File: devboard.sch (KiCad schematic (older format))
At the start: 112 parts, among them J1 USB_B, K1 HF3FA-012-ZTF, K2 HF3FA-012-ZTF

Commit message: Switches and buttons finished
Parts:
- added J?: Switches, symbol Connector_Generic:Conn_01x08
- K1, K2, K?: symbol hello-there:HF3FA-012-ZTF -> devboard-rescue:HF3FA-012-ZTF-hello-there
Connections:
- net S1: now also J?.1 (Pin_1)
- net S2: now also J?.2 (Pin_2)
- net S3: now also J?.3 (Pin_3)
- net S4: now also J?.4 (Pin_4)
- net S5: now also J?.5 (Pin_5)
- net S6: now also J?.6 (Pin_6)
- net S7: now also J?.7 (Pin_7)
- net S8: now also J?.8 (Pin_8)
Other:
- note added: "Switches"
- moved on the sheet: C?, R?, SW?

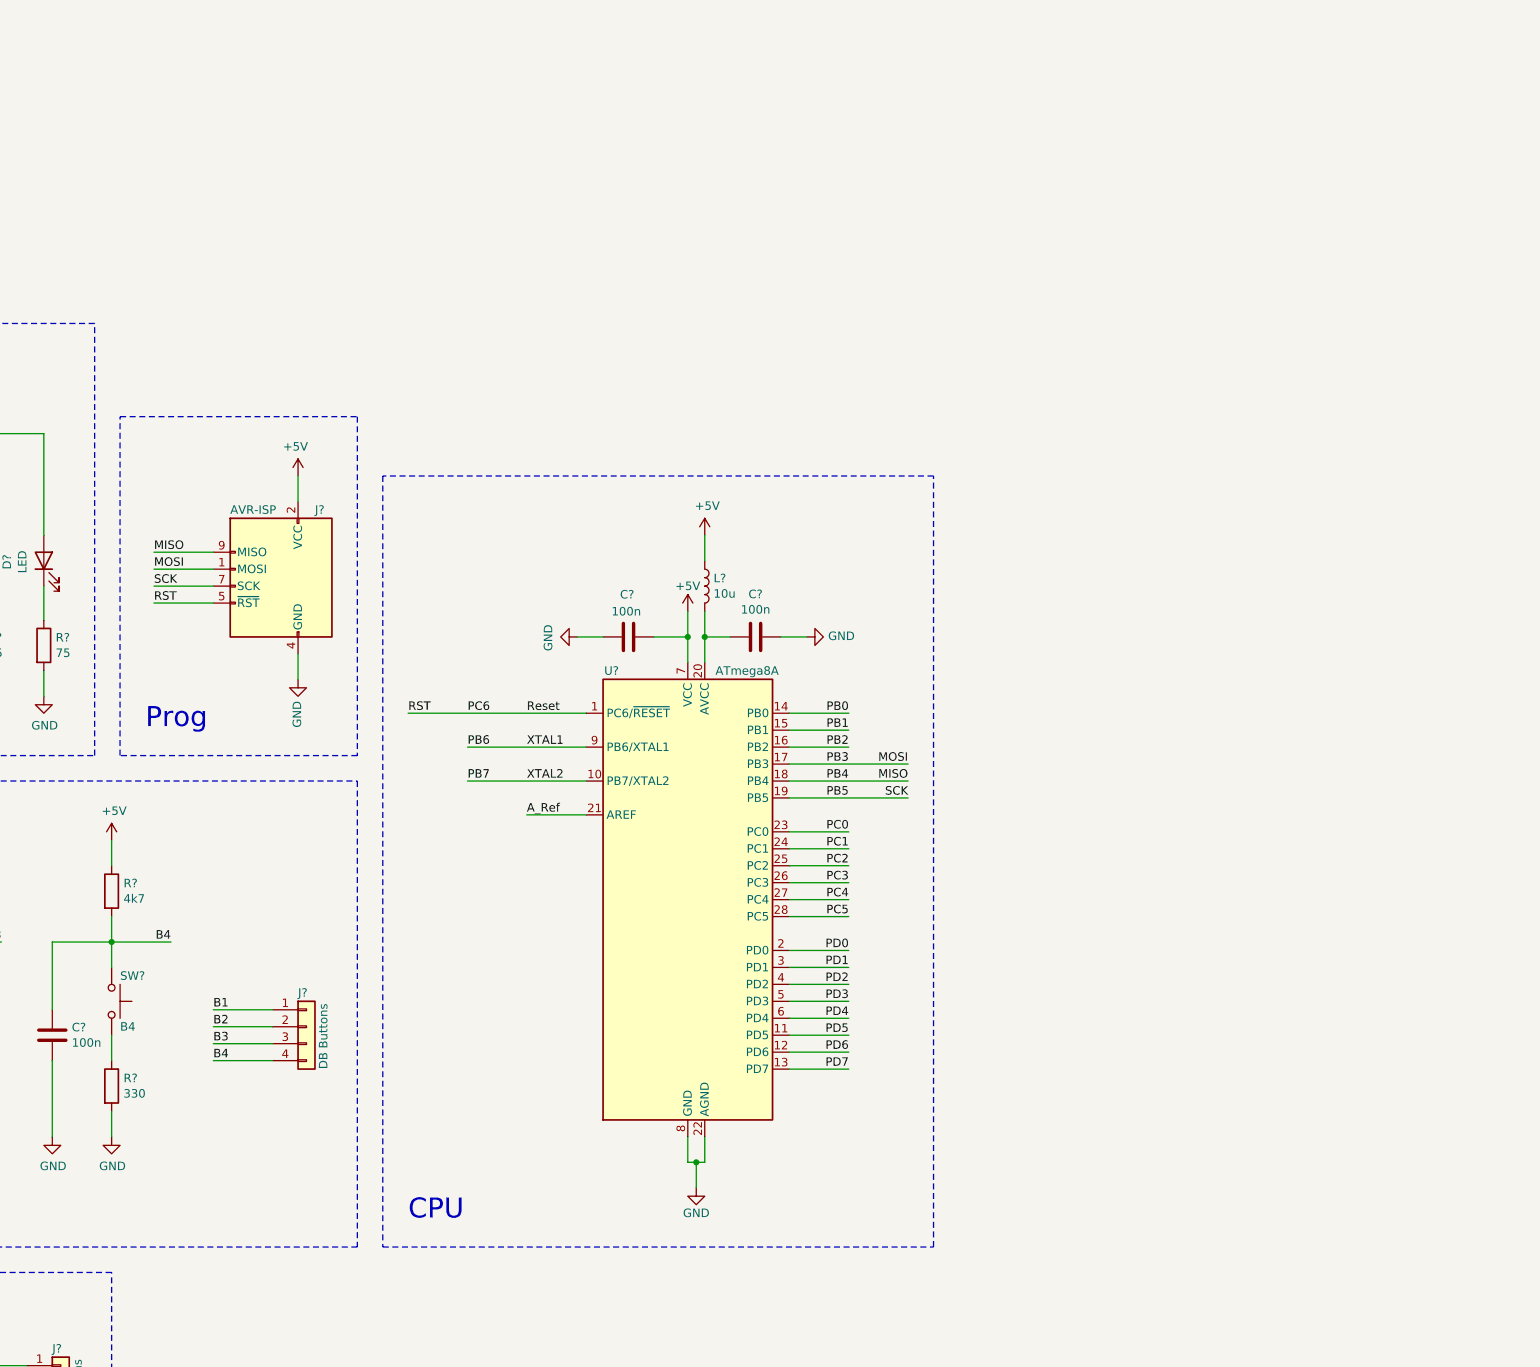
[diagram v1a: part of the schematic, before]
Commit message: Pots + rgb
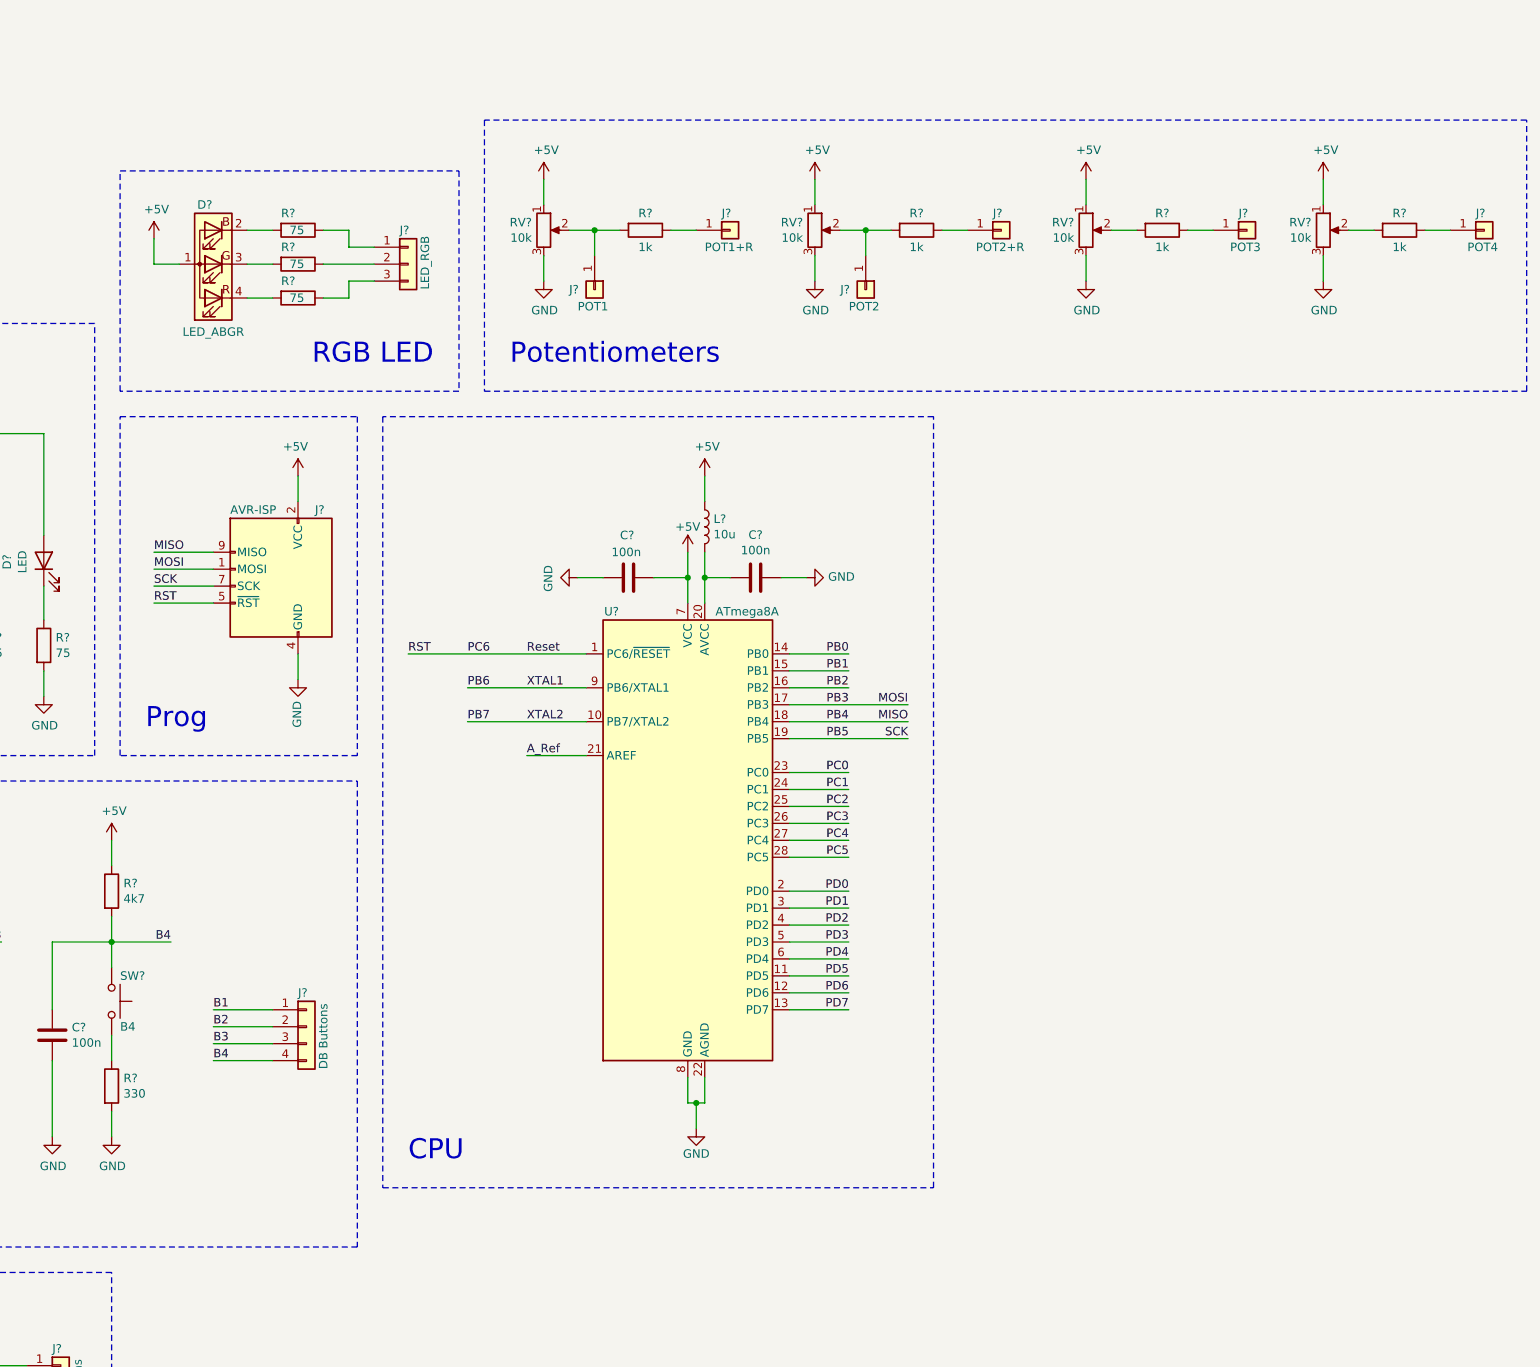
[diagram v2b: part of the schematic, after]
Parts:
- added D?: LED_ABGR, symbol Device:LED_ABGR
- added J?: LED_RGB, symbol Connector_Generic:Conn_01x03
- added J?: POT4, symbol Connector_Generic:Conn_01x01
- added J?: POT3, symbol Connector_Generic:Conn_01x01
- added J?: POT2+R, symbol Connector_Generic:Conn_01x01
- added J?: POT2, symbol Connector_Generic:Conn_01x01
- added J?: POT1+R, symbol Connector_Generic:Conn_01x01
- added J?: POT1, symbol Connector_Generic:Conn_01x01
- added R? (x3): 75, symbol Device:R
- added R? (x4): 1k, symbol Device:R
- added RV? (x4): 10k, symbol Device:R_POT
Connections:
- net +5V: now also D?.1 (A), RV?.1, RV?.1, RV?.1, RV?.1
- net GND: now also RV?.3, RV?.3, RV?.3, RV?.3
- new net: D?.2 (BK), R?.2
- new net: D?.3 (GK), R?.2
- new net: D?.4 (RK), R?.2
- new net: J?.1 (Pin_1), R?.1 (x5)
- new net: J?.2 (Pin_2), R?.1
- new net: J?.3 (Pin_3), R?.1
- new net: R?.2, RV?.2 (x2)
- new net: J?.1 (Pin_1), R?.2, RV?.2 (x2)
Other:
- note added: "Potentiometers"
- note added: "RGB LED"
- moved on the sheet: C?, L?, U?
